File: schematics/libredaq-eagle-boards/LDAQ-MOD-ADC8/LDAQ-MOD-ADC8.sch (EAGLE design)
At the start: 17 parts, among them CON1 BOARD, IC1 24C01ASN, J1 ADC[0-7], SW1 SW_DIP-4, U1 AD7606

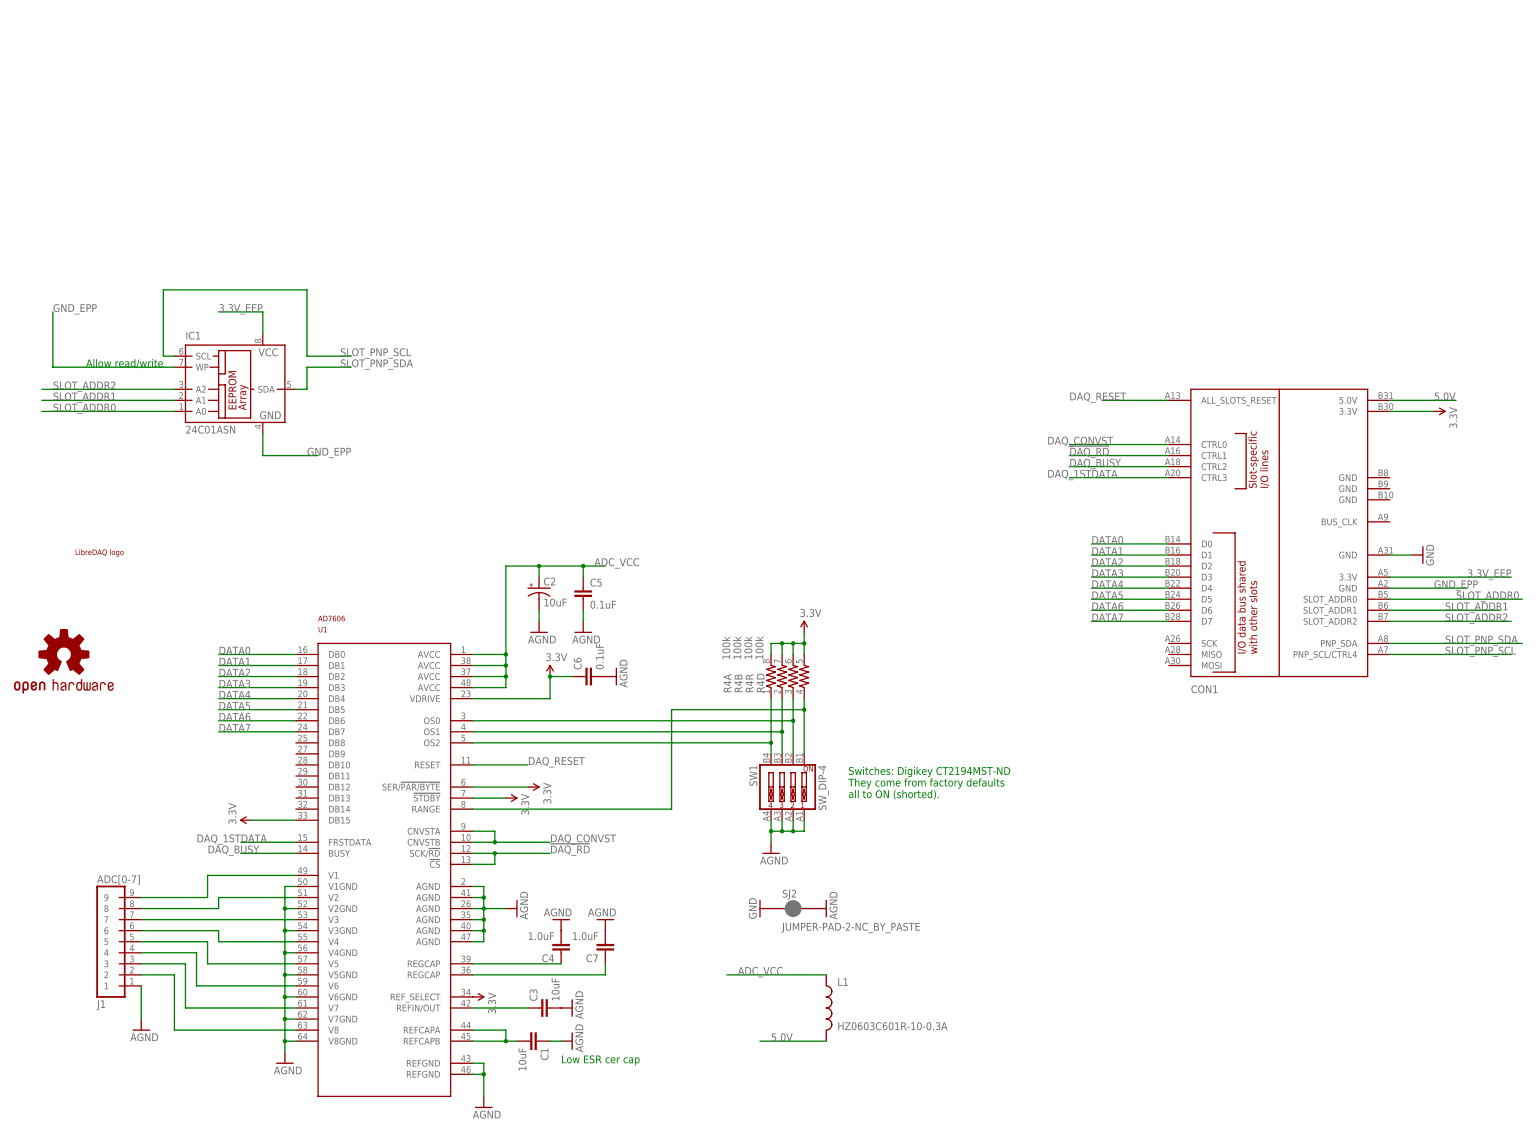
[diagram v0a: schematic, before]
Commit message: update adc8 board
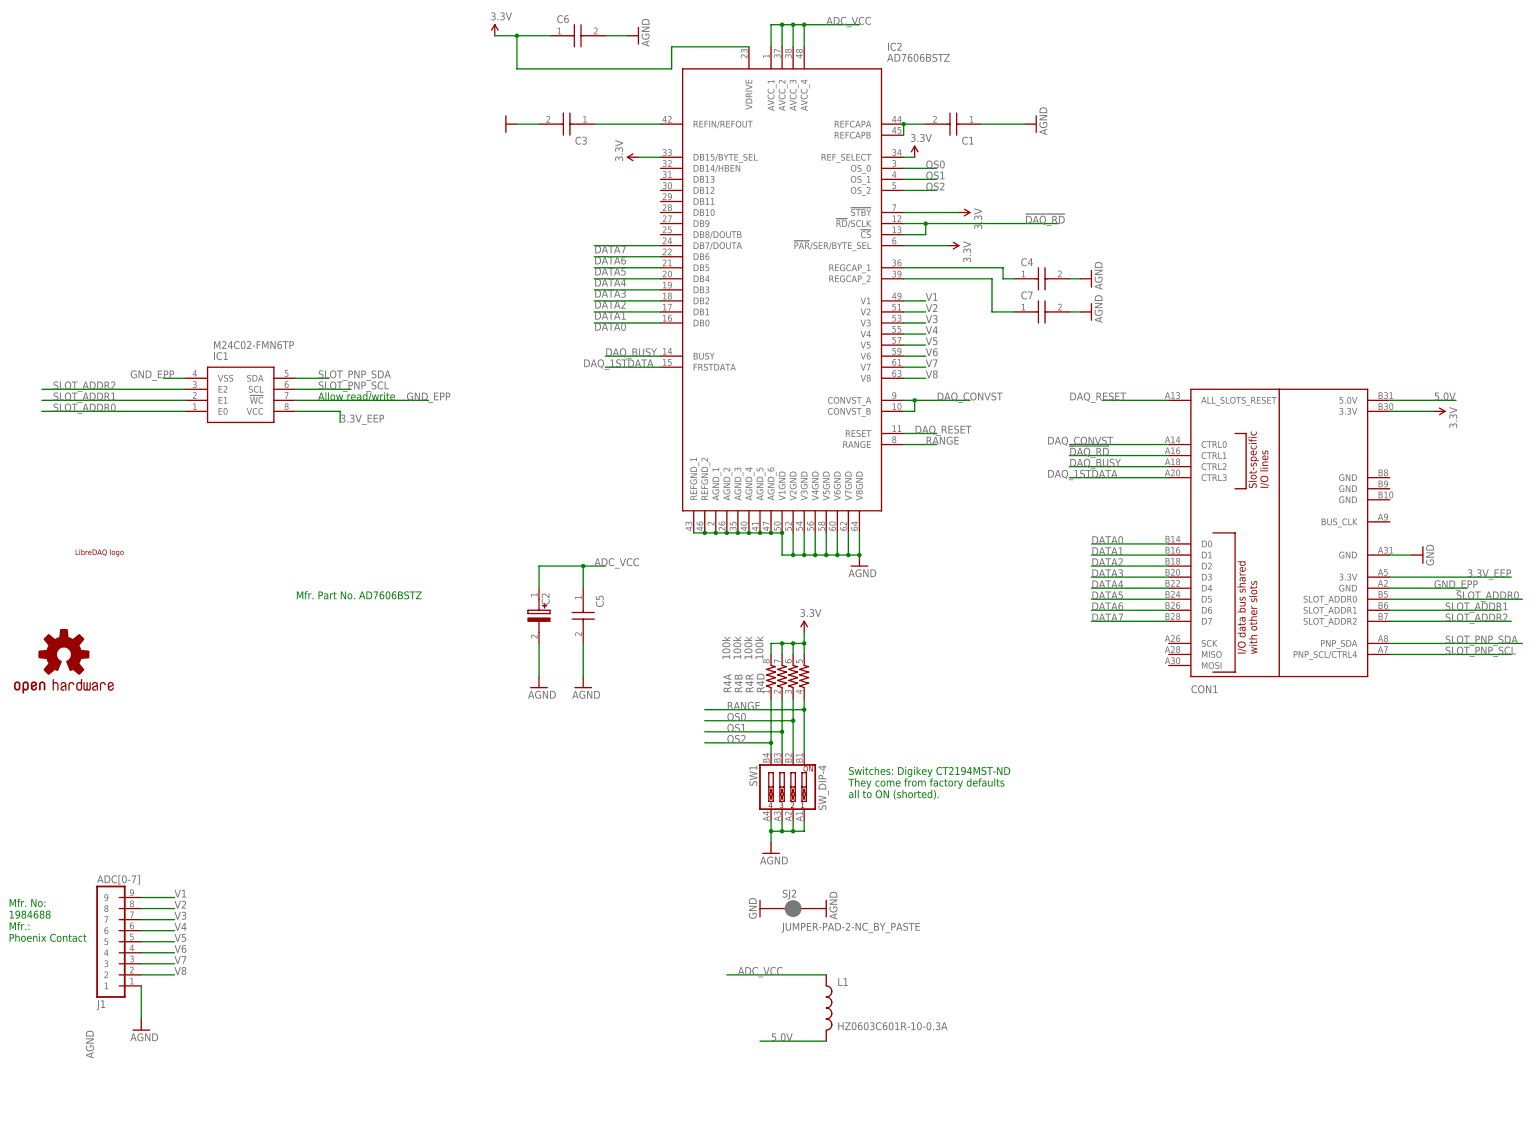
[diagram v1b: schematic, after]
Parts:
- removed U1: AD7606, libredaq-comps:AD7606
- added IC2: AD7606BSTZ, SamacSys_Parts:AD7606BSTZ
- C1, C3: device SparkFun-Capacitors:10UF-6.3V-20%(0603) -> LMK105BJ225KV-F:LMK105BJ225KV-F
- C2: device SparkFun-Capacitors:10UF-16V-10%(TANT) -> TAJB226M010RNJ:TAJB226M010RNJ
- C4, C7: device SparkFun-Capacitors:1.0UF-16V-10%(0603) -> LMK105BJ225KV-F:LMK105BJ225KV-F
- C5, C6: device SparkFun-Capacitors:0.1UF-25V(+80/-20%)(0603) -> 885012105010:885012105010
- IC1: value 24C01ASN -> M24C02-FMN6TP; device libredaq-comps:24C01ASN -> SamacSys_Parts:M24C02-FMN6TP
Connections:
- removed net N$17: R4B.1, SW1.B3, U1.OS1
- removed net N$18: R4A.1, SW1.B4, U1.OS2
- removed net N$33: C4.1, U1.REGCAP@39
- removed net N$34: C7.1, U1.REGCAP@36
- removed net N$36: J1.9, U1.V1
- removed net N$37: J1.8, U1.V2
- removed net N$38: J1.7, U1.V3
- removed net N$39: J1.6, U1.V4
- removed net N$40: J1.5, U1.V5
- removed net N$41: J1.4, U1.V6
- removed net N$42: J1.3, U1.V7
- removed net N$43: J1.2, U1.V8
- removed net N$44: C1.2, U1.REFCAPA, U1.REFCAPB
- removed net N$5: R4R.1, SW1.B2, U1.OS0
- new net N$1: C1.2, IC2.REFCAPA, IC2.REFCAPB
- new net N$2: C4.1, IC2.REGCAP_1
- new net OS0: IC2.OS_0, R4R.1, SW1.B2
- new net OS1: IC2.OS_1, R4B.1, SW1.B3
- new net OS2: IC2.OS_2, R4A.1, SW1.B4
- new net RANGE: IC2.RANGE, R4D.1, SW1.B1
- new net V1: IC2.V1, J1.9
- new net V2: IC2.V2, J1.8
- new net V3: IC2.V3, J1.7
- new net V4: IC2.V4, J1.6
- new net V5: IC2.V5, J1.5
- new net V6: IC2.V6, J1.4
- new net V7: IC2.V7, J1.3
- new net V8: IC2.V8, J1.2
- net !DAQ_RD: now also IC2.!CS, IC2.!RD!/SCLK; no longer U1.!CS, U1.SCK/!RD
- net 3.3V: now also IC2.!PAR!/SER/BYTE_SEL, IC2.!STBY, IC2.DB15/BYTE_SEL, IC2.REF_SELECT, IC2.VDRIVE; no longer U1.!STDBY, U1.DB15, U1.REF_SELECT, U1.SER/!PAR/BYTE, U1.VDRIVE
- net ADC_VCC: now also IC2.AVCC_1, IC2.AVCC_2, IC2.AVCC_3, IC2.AVCC_4; no longer U1.AVCC@1, U1.AVCC@37, U1.AVCC@38, U1.AVCC@48
- net AGND: now also IC2.AGND_1, IC2.AGND_2, IC2.AGND_3, IC2.AGND_4, IC2.AGND_5, IC2.AGND_6, IC2.REFGND_1, IC2.REFGND_2, IC2.V1GND, IC2.V2GND, IC2.V3GND, IC2.V4GND, IC2.V5GND, IC2.V6GND, IC2.V7GND, IC2.V8GND; no longer U1.AGND@2, U1.AGND@26, U1.AGND@35, U1.AGND@40, U1.AGND@41, U1.AGND@47, U1.REFGND@43, U1.REFGND@46, U1.V1GND, U1.V2GND, U1.V3GND, U1.V4GND, U1.V5GND, U1.V6GND, U1.V7GND, U1.V8GND
- net DAQ_1STDATA: now also IC2.FRSTDATA; no longer U1.FRSTDATA
- net DAQ_BUSY: now also IC2.BUSY; no longer U1.BUSY
- net DAQ_CONVST: now also IC2.CONVST_A, IC2.CONVST_B; no longer U1.CNVSTA, U1.CNVSTB
- net DAQ_RESET: now also IC2.RESET; no longer U1.RESET
- net DATA0: now also IC2.DB0; no longer U1.DB0
- net DATA1: now also IC2.DB1; no longer U1.DB1
- net DATA2: now also IC2.DB2; no longer U1.DB2
- net DATA3: now also IC2.DB3; no longer U1.DB3
- net DATA4: now also IC2.DB4; no longer U1.DB4
- net DATA5: now also IC2.DB5; no longer U1.DB5
- net DATA6: now also IC2.DB6; no longer U1.DB6
- net DATA7: now also IC2.DB7/DOUTA; no longer U1.DB7
- net GND_EPP: now also IC1.!WC, IC1.VSS; no longer IC1.GND, IC1.WP
- net N$3: now also C7.1, IC2.REGCAP_2; no longer R4D.1, SW1.B1, U1.RANGE
- net N$35: now also IC2.REFIN/REFOUT; no longer U1.REFIN/OUT
- net SLOT_ADDR0: now also IC1.E0; no longer IC1.A0
- net SLOT_ADDR1: now also IC1.E1; no longer IC1.A1
- net SLOT_ADDR2: now also IC1.E2; no longer IC1.A2
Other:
- note added: "Mfr. No: 1984688 Mfr.: Phoenix Contact"
- note added: "Mfr. Part No. AD7606BSTZ"
- note removed: "Low ESR cer cap"
